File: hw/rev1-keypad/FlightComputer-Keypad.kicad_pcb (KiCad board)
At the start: 2 copper layers, 36 x 148 mm, 37 parts, among them J1 Conn_02x20_Odd_Even, SW1 SW_Push, SW2 SW_Push, SW3 SW_Push, SW4 SW_Push, SW5 SW_Push, SW6 SW_Push, SW7 SW_Push, SW8 SW_Push, SW9 SW_Push

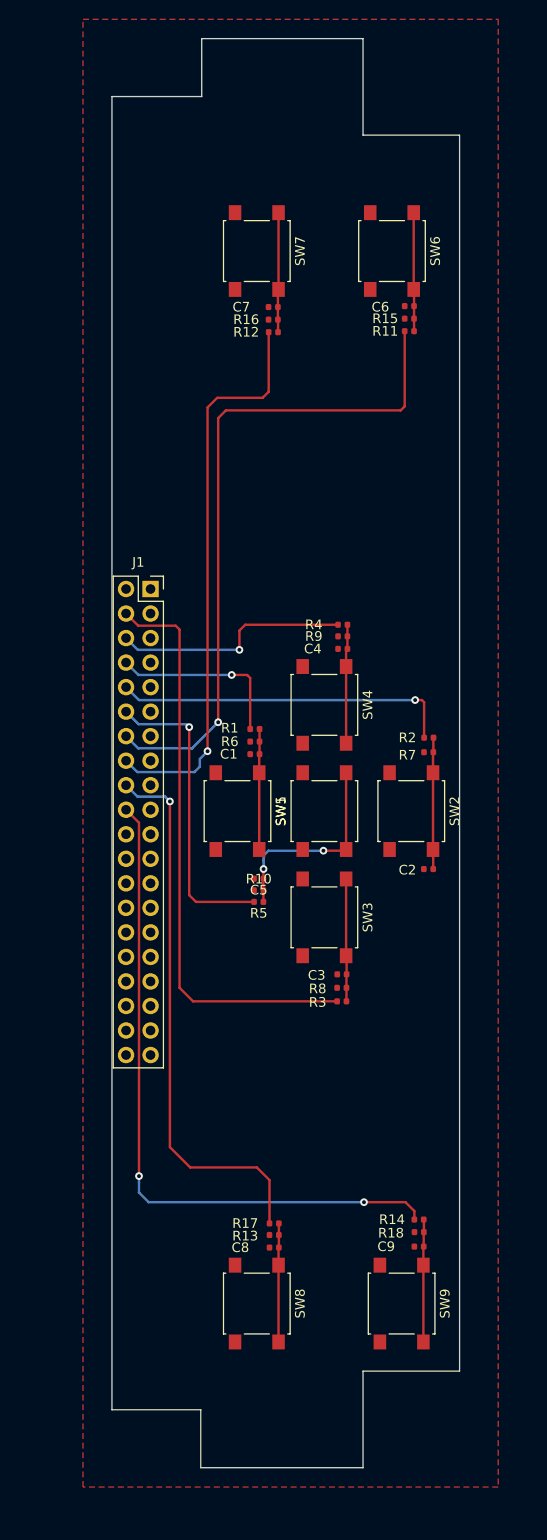
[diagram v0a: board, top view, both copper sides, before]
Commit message: ...
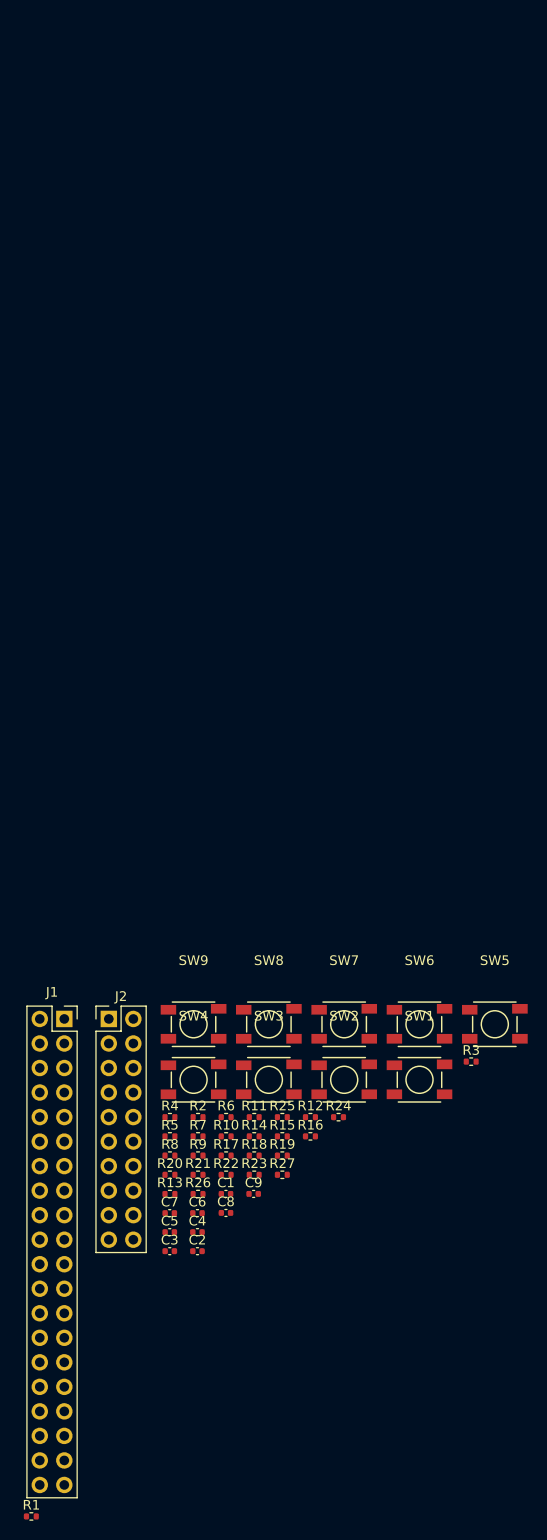
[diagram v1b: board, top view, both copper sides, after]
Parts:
- added J2: Conn_02x10_Odd_Even, Connector_PinHeader_2.54mm:PinHeader_2x10_P2.54mm_Vertical, F.Cu at (49.7, 131.5)
- added R19: 100K, Resistor_SMD:R_0402_1005Metric, F.Cu at (67.6, 145.7)
- added R20: 100K, Resistor_SMD:R_0402_1005Metric, F.Cu at (56.0, 147.7)
- added R21: 33R, Resistor_SMD:R_0402_1005Metric, F.Cu at (58.9, 147.7)
- added R22: 33R, Resistor_SMD:R_0402_1005Metric, F.Cu at (61.8, 147.7)
- added R23: 33R, Resistor_SMD:R_0402_1005Metric, F.Cu at (64.7, 147.7)
- added R24: 33R, Resistor_SMD:R_0402_1005Metric, F.Cu at (73.5, 141.7)
- added R25: 33R, Resistor_SMD:R_0402_1005Metric, F.Cu at (67.6, 141.7)
- added R26: 33R, Resistor_SMD:R_0402_1005Metric, F.Cu at (58.9, 149.7)
- added R27: 100K, Resistor_SMD:R_0402_1005Metric, F.Cu at (67.6, 147.7)
- SW1, SW2, SW3, SW4, SW5, SW6, SW7, SW8, SW9: footprint Button_Switch_SMD:SW_SPST_B3S-1000 -> FlightComputer_Library:SW_SPST_PTS647
- moved C6 96.5 mm to (58.9, 151.6), turned to 0 degrees
- moved C7 94.4 mm to (56.0, 151.6), turned to 0 degrees
- moved R15 85.7 mm to (67.6, 143.7)
- moved R1 84.8 mm to (41.7, 183.0), turned to 0 degrees
- moved R16 84.7 mm to (70.6, 143.7)
- moved R11 83.0 mm to (64.7, 141.7), turned to 0 degrees
- moved R12 81.4 mm to (70.6, 141.7), turned to 0 degrees
- moved SW7 80.6 mm to (74.0, 132.1), turned to 0 degrees
- moved SW6 80.1 mm to (81.8, 132.1), turned to 0 degrees
- moved C4 62.3 mm to (58.9, 153.6), turned to 0 degrees
- moved R9 55.8 mm to (58.9, 145.7)
- moved R4 54.0 mm to (56.0, 141.7), turned to 0 degrees
- moved R7 46.4 mm to (58.9, 143.7)
- moved C2 46.2 mm to (58.9, 155.6), turned to 0 degrees
- moved R2 46.0 mm to (58.9, 141.7), turned to 0 degrees
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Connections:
- J1 pad 1: Net-(J1-Pad1) -> VCC_MCU
- J1 pad 11: Net-(J1-Pad11) -> /KEY_POWER
- J1 pad 13: Net-(J1-Pad13) -> /KEY_ENTER
- J1 pad 15: Net-(J1-Pad15) -> /KEY_ESCAPE
- J1 pad 17: Net-(J1-Pad17) -> /KEY_FUNC1
- J1 pad 19: Net-(J1-Pad19) -> /KEY_FUNC2
- J1 pad 2: VCC_PERIH -> VCC_MCU
- J1 pad 27: Net-(J1-Pad27) -> /TRST
- J1 pad 28: Net-(J1-Pad28) -> /TRST
- J1 pad 29: Net-(J1-Pad29) -> /TDI
- J1 pad 3: Net-(J1-Pad3) -> /KEY_LEFT
- J1 pad 30: Net-(J1-Pad30) -> /TDI
- J1 pad 31: Net-(J1-Pad31) -> /TMS
- J1 pad 32: Net-(J1-Pad32) -> /TMS
- J1 pad 33: Net-(J1-Pad33) -> /TCLK
- J1 pad 34: Net-(J1-Pad34) -> /TCLK
- J1 pad 35: Net-(J1-Pad35) -> /TDO
- J1 pad 36: Net-(J1-Pad36) -> /TDO
- J1 pad 37: Net-(J1-Pad37) -> /nRESET
- J1 pad 38: Net-(J1-Pad38) -> /nRESET
- J1 pad 39: Net-(J1-Pad39) -> GND
- J1 pad 5: Net-(J1-Pad5) -> /KEY_RIGHT
- J1 pad 7: Net-(J1-Pad7) -> /KEY_UP
- J1 pad 9: Net-(J1-Pad9) -> /KEY_DOWN
- SW1 pad 2: VCC_PERIH -> VCC_MCU
- SW2 pad 2: VCC_PERIH -> VCC_MCU
- SW3 pad 2: VCC_PERIH -> VCC_MCU
- SW4 pad 2: VCC_PERIH -> VCC_MCU
- SW5 pad 1: VCC_PERIH -> VCC_MCU
- SW6 pad 2: VCC_PERIH -> VCC_MCU
- SW7 pad 2: VCC_PERIH -> VCC_MCU
- SW8 pad 2: VCC_PERIH -> VCC_MCU
- SW9 pad 2: VCC_PERIH -> VCC_MCU
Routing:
- net /KEY_FUNC2: track 70.4 -> 0.00 mm, vias 2 -> 0
- net /KEY_ENTER: track 70.3 -> 0.00 mm, vias 1 -> 0
- net /KEY_LEFT: track 60.2 -> 0.00 mm
- net /KEY_ESCAPE: track 59.1 -> 0.00 mm, vias 1 -> 0
- net /KEY_FUNC1: track 57.3 -> 0.00 mm, vias 1 -> 0
- net /KEY_DOWN: track 35.2 -> 0.00 mm, vias 1 -> 0
- net /KEY_POWER: track 31.6 -> 0.00 mm, vias 1 -> 0
- net /KEY_RIGHT: track 24.7 -> 0.00 mm, vias 1 -> 0
- net Net-(C5-Pad1): track 21.6 -> 0.00 mm, vias 2 -> 0
- net /KEY_UP: track 18.8 -> 0.00 mm, vias 1 -> 0
- net Net-(C2-Pad1): track 13.6 -> 0.00 mm
- net Net-(C9-Pad1): track 12.7 -> 0.00 mm
- net Net-(C3-Pad1): track 12.7 -> 0.00 mm
- net Net-(C1-Pad1): track 12.5 -> 0.00 mm
- net Net-(C7-Pad1): track 12.4 -> 0.00 mm
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- removed copper zone on F.Cu, net GND
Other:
- board outline removed
- rule pad_to_mask_clearance: 0.05 -> 0
